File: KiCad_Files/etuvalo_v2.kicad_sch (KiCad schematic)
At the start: 38 parts, among them J1 Conn_01x06, J10 Conn_01x01, J11 Conn_01x01, J2 Conn_01x02, J3 Conn_01x02, J4 Conn_01x03, J5 Conn_01x03, J6 Conn_01x03, J7 Conn_01x01, J8 Conn_01x01, J9 Conn_01x01, U1 ATtiny814-SS, U2 AMS1117-5.0

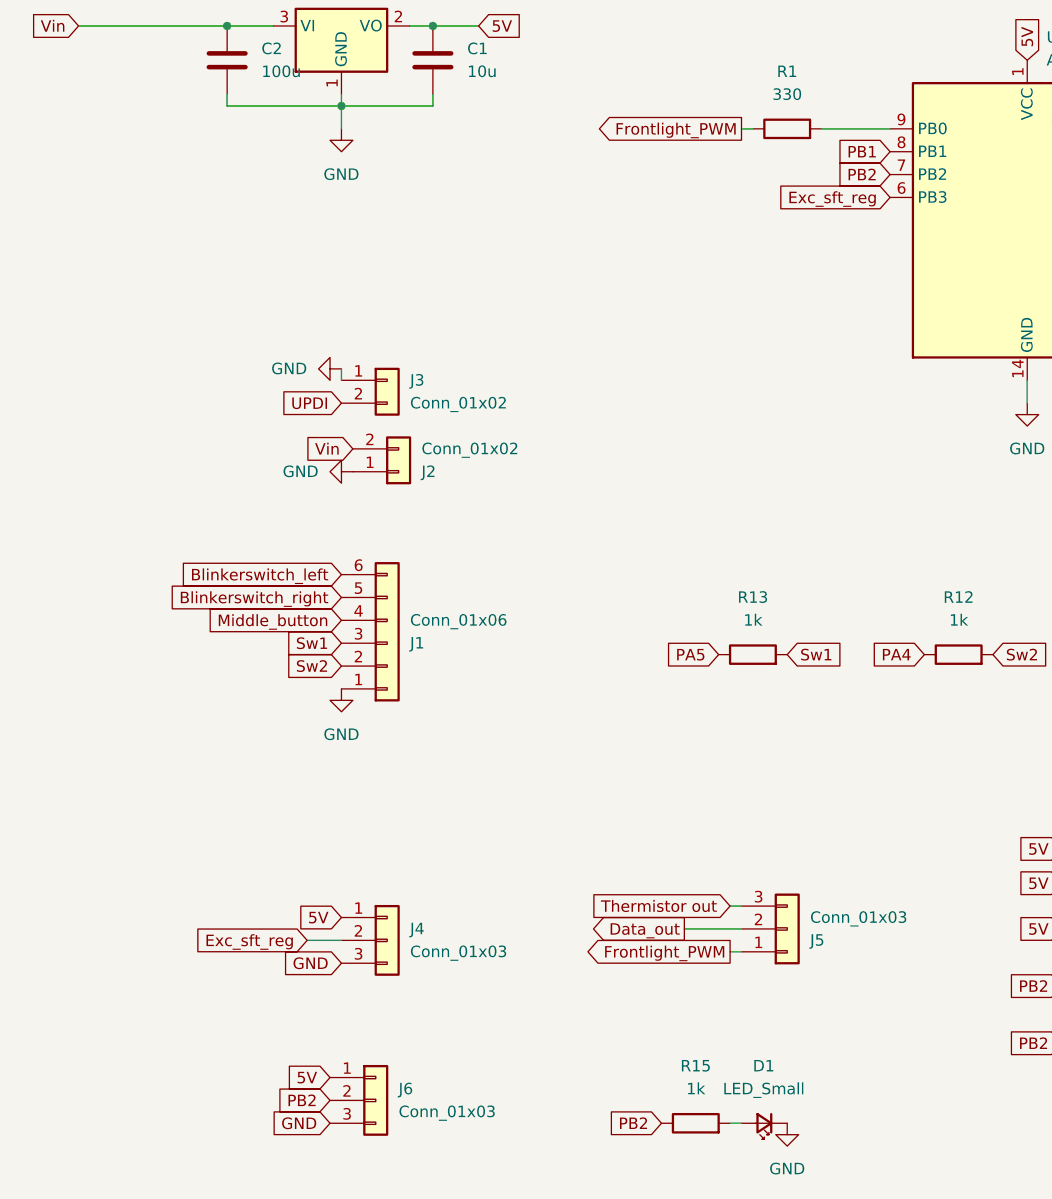
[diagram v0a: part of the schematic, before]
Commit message: Changes
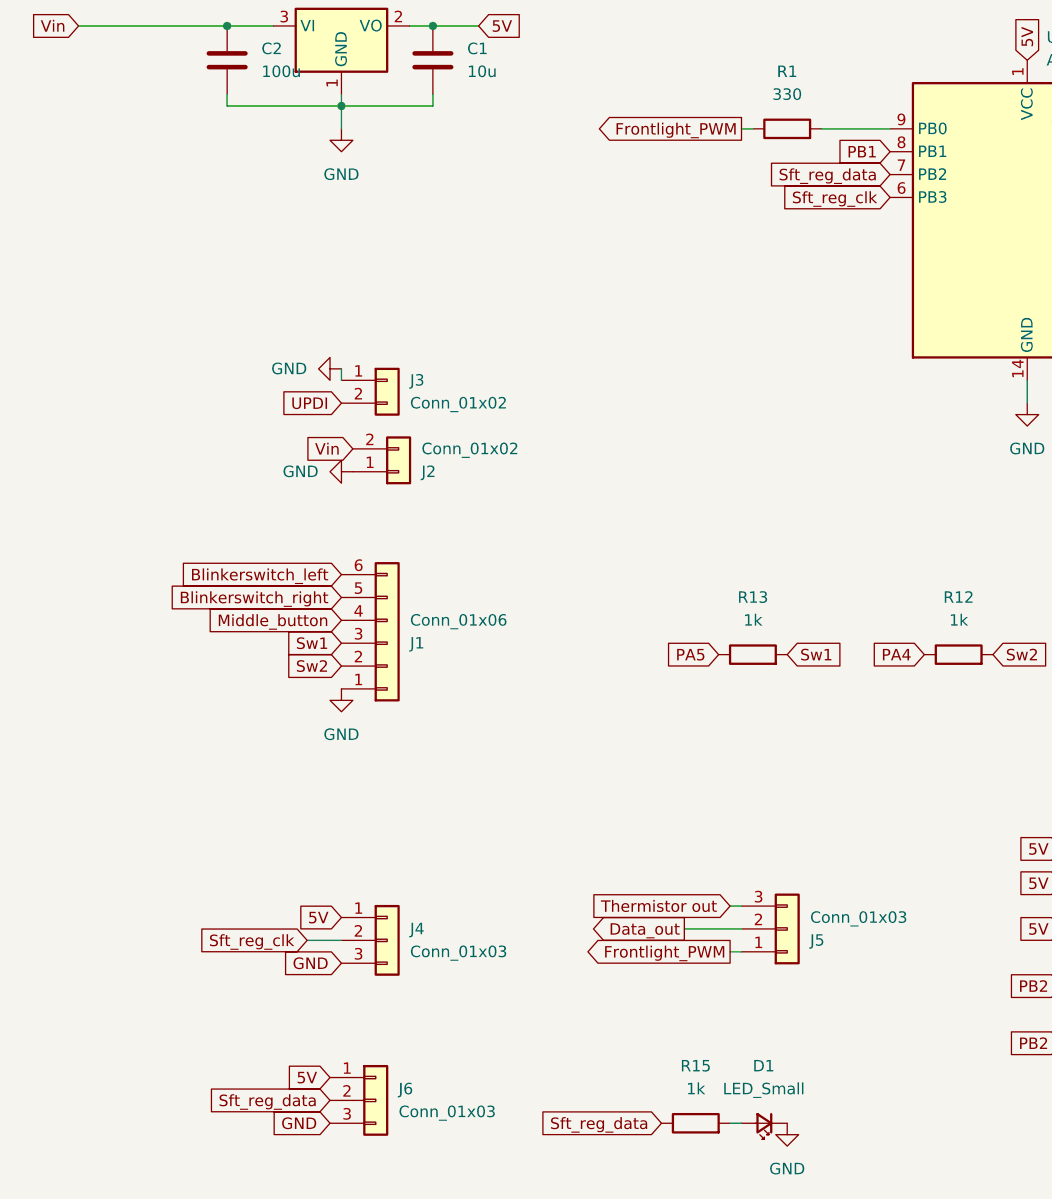
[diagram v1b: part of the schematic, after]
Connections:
- net PB2: no longer J6.2 (Pin_2), R15.1, U1.7 (PB2)
- net Exc_sft_reg renamed Sft_reg_clk
- new net Sft_reg_data: J6.2 (Pin_2), R15.1, U1.7 (PB2)
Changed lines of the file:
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@@
 		)
 	)
-	(global_label "PB2"
+	(global_label "Sft_reg_data"
 		(shape input)
 		(at 91.44 186.69 180)
@@
 		)
 		(property "Intersheetrefs" "${INTERSHEET_REFS}"
-			(at 84.7053 186.69 0)
+			(at 76.6622 186.69 0)
 			(effects
 				(font
@@
 		)
 	)
-	(global_label "Exc_sft_reg"
+	(global_label "Sft_reg_clk"
 		(shape input)
 		(at 116.84 83.82 180)
@@
 		)
 		(property "Intersheetrefs" "${INTERSHEET_REFS}"
-			(at 103.1506 83.82 0)
+			(at 103.453 83.82 0)
 			(effects
 				(font
@@
 		)
 	)
+	(global_label "Sft_reg_clk"
+		(shape input)
+		(at 52.07 166.37 180)
+		(fields_autoplaced yes)
+		(effects
+			(font
+				(size 1.27 1.27)
+			)
+			(justify right)
+		)
+		(property "Intersheetrefs" "${INTERSHEET_REFS}"
+			(at 38.683 166.37 0)
+			(effects
+				(font
+					(size 1.27 1.27)
+				)
+				(justify right)
+				(hide yes)
+			)
+		)
+	)
 	(global_label "5V"
 		(shape input)
@@
 		)
 	)
-	(global_label "PB2"
-		(shape input)
-		(at 116.84 81.28 180)
-		(fields_autoplaced yes)
-		(effects
-			(font
-				(size 1.27 1.27)
-			)
-			(justify right)
-		)
-		(property "Intersheetrefs" "${INTERSHEET_REFS}"
-			(at 110.1053 81.28 0)
-			(effects
-				(font
-					(size 1.27 1.27)
-				)
-				(justify right)
-				(hide yes)
-			)
-		)
-	)
 	(global_label "Sw2"
 		(shape input)
@@
 				)
 				(justify left)
-				(hide yes)
-			)
-		)
-	)
-	(global_label "PB2"
-		(shape input)
-		(at 54.61 184.15 180)
-		(fields_autoplaced yes)
-		(effects
-			(font
-				(size 1.27 1.27)
-			)
-			(justify right)
-		)
-		(property "Intersheetrefs" "${INTERSHEET_REFS}"
-			(at 47.8753 184.15 0)
-			(effects
-				(font
-					(size 1.27 1.27)
-				)
-				(justify right)
 				(hide yes)
 			)
@@
 		)
 	)
+	(global_label "Sft_reg_data"
+		(shape input)
+		(at 116.84 81.28 180)
+		(fields_autoplaced yes)
+		(effects
+			(font
+				(size 1.27 1.27)
+			)
+			(justify right)
+		)
+		(property "Intersheetrefs" "${INTERSHEET_REFS}"
+			(at 102.0622 81.28 0)
+			(effects
+				(font
+					(size 1.27 1.27)
+				)
+				(justify right)
+				(hide yes)
+			)
+		)
+	)
 	(global_label "5V"
 		(shape input)
@@
 		)
 	)
-	(global_label "Exc_sft_reg"
-		(shape input)
-		(at 52.07 166.37 180)
-		(fields_autoplaced yes)
-		(effects
-			(font
-				(size 1.27 1.27)
-			)
-			(justify right)
-		)
-		(property "Intersheetrefs" "${INTERSHEET_REFS}"
-			(at 38.3806 166.37 0)
-			(effects
-				(font
-					(size 1.27 1.27)
-				)
-				(justify right)
-				(hide yes)
-			)
-		)
-	)
 	(global_label "Blinkerswitch_left"
 		(shape input)
@@
 			(effects
 				(font
+					(size 1.27 1.27)
+				)
+				(justify right)
+				(hide yes)
+			)
+		)
+	)
+	(global_label "Sft_reg_data"
+		(shape input)
+		(at 54.61 184.15 180)
+		(fields_autoplaced yes)
+		(effects
+			(font
+				(size 1.27 1.27)
+			)
+			(justify right)
+		)
+		(property "Intersheetrefs" "${INTERSHEET_REFS}"
+			(at 39.8322 184.15 0)
+			(effects
+				(font
